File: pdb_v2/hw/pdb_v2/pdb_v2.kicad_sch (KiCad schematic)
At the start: 71 parts, among them J1 XT30-M_Ver, J2 JST-PH_01x02, J3 Conn_01x06_Pin, J5 JST-PH_01x02, J6 Conn_01x03, J7 Conn_01x03, J8 Conn_01x04, Q1 60Vds, SW1 SW_Push, SW2 SW_Push, U1 LMR51635XFDDCR, U2 ESP32-WROOM-32, U3 AP63203WU-7

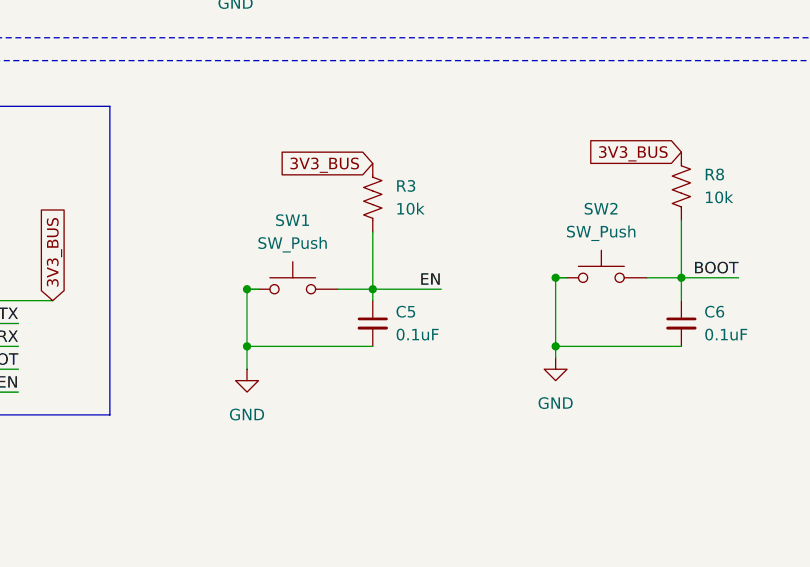
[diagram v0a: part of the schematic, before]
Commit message: Sent to Matthew for review
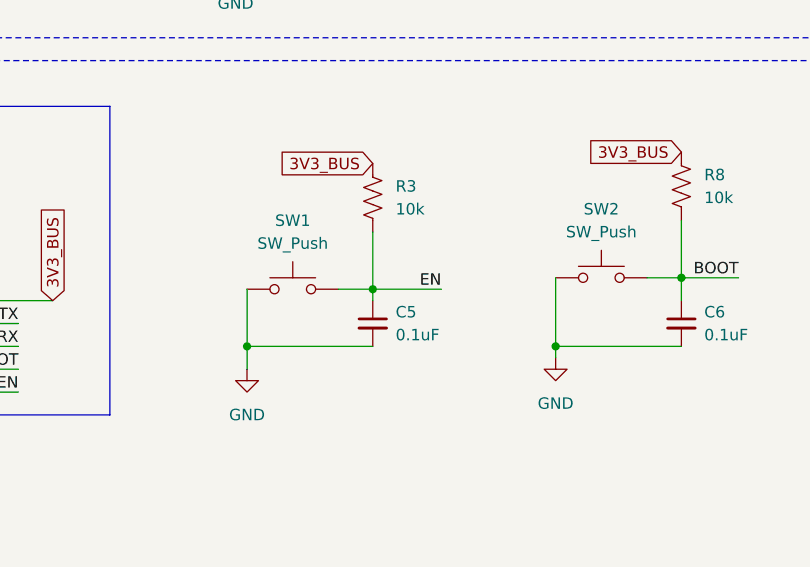
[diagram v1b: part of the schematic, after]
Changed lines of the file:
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@@
-	)
-	(junction
-		(at 81.28 203.2)
-		(diameter 0)
-		(color 0 0 0 0)
 	)
 	(junction
@@
 	)
 	(junction
-		(at 115.57 201.93)
-		(diameter 0)
-		(color 0 0 0 0)
-	)
-	(junction
 		(at 129.54 201.93)
 		(diameter 0)
@@
 	(wire
 		(pts
-			(xy 81.28 203.2) (xy 82.55 203.2)
-		)
-		(stroke
-			(width 0)
-			(type default)
-		)
-	)
-	(wire
-		(pts
 			(xy 331.47 38.1) (xy 331.47 46.99)
 		)
@@
 		)
 		(stroke
-			(width 0)
-			(type default)
-		)
-	)
-	(wire
-		(pts
-			(xy 115.57 201.93) (xy 116.84 201.93)
-		)
-		(stroke
